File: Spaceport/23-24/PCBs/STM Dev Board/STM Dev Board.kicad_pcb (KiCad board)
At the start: 2 copper layers, 61 x 33 mm, 5 parts, among them J1 693023010811, J2 614004184726, U2 IS66WVS4M8BLL-104NLI, U3 W25X40CLSNIG

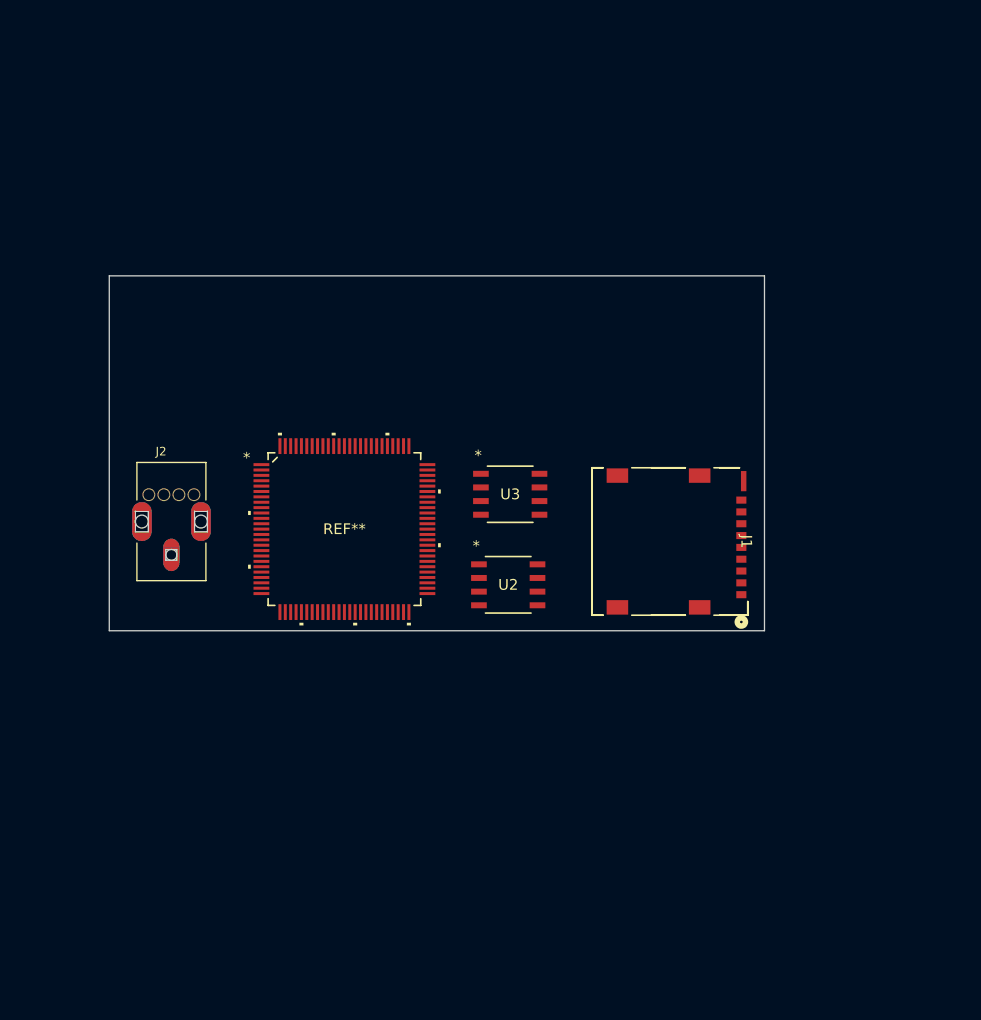
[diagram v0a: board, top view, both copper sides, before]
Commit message: commit 3
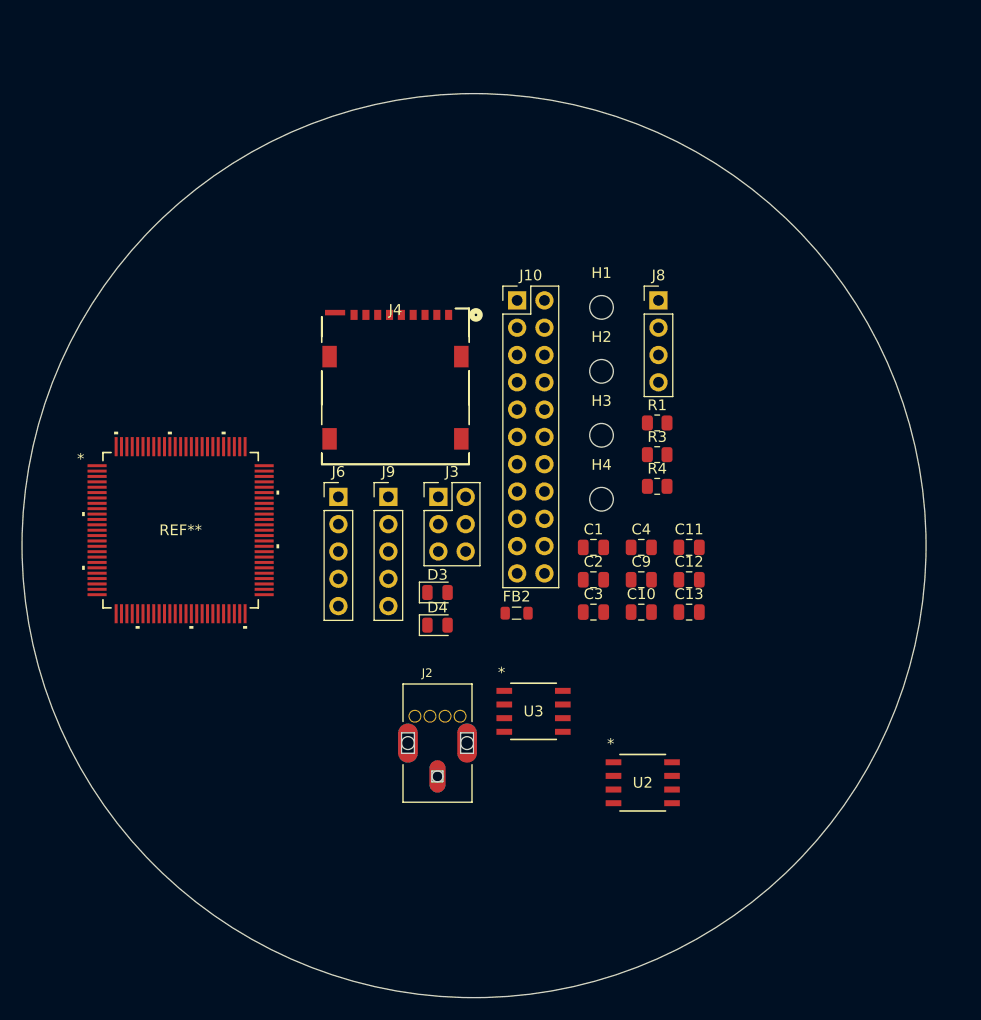
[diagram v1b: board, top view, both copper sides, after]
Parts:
- removed J1: 693023010811, 693023010811:CONN9_3010811_WRE
- removed the REF** at (137.2, 93.9)
- added C1: 100n, Capacitor_SMD:C_0805_2012Metric, F.Cu at (160.3, 95.6)
- added C10: 1u, Capacitor_SMD:C_0805_2012Metric, F.Cu at (164.8, 101.6)
- added C11: 10n, Capacitor_SMD:C_0805_2012Metric, F.Cu at (169.2, 95.6)
- added C12: 100n, Capacitor_SMD:C_0805_2012Metric, F.Cu at (169.2, 98.6)
- added C13: 1u, Capacitor_SMD:C_0805_2012Metric, F.Cu at (169.2, 101.6)
- added C2: 100n, Capacitor_SMD:C_0805_2012Metric, F.Cu at (160.3, 98.6)
- added C3: 100n, Capacitor_SMD:C_0805_2012Metric, F.Cu at (160.3, 101.6)
- added C4: 100n, Capacitor_SMD:C_0805_2012Metric, F.Cu at (164.8, 95.6)
- added C9: 1u, Capacitor_SMD:C_0805_2012Metric, F.Cu at (164.8, 98.6)
- added D3: RADIO_LED, LED_SMD:LED_0805_2012Metric, F.Cu at (145.8, 99.8)
- added D4: RADIO_LED, LED_SMD:LED_0805_2012Metric, F.Cu at (145.8, 102.8)
- added FB2: 120R, Inductor_SMD:L_0805_2012Metric, F.Cu at (153.2, 101.7)
- added H1: MountingHole, MountingHole:MountingHole_2.2mm_M2, F.Cu at (161.1, 73.2)
- added H2: MountingHole, MountingHole:MountingHole_2.2mm_M2, F.Cu at (161.1, 79.2)
- added H3: MountingHole, MountingHole:MountingHole_2.2mm_M2, F.Cu at (161.1, 85.2)
- added H4: MountingHole, MountingHole:MountingHole_2.2mm_M2, F.Cu at (161.1, 91.1)
- added J10: GPIO, Connector_PinHeader_2.54mm:PinHeader_2x11_P2.54mm_Vertical, F.Cu at (153.2, 72.6)
- added J3: SPI, Connector_PinHeader_2.54mm:PinHeader_2x03_P2.54mm_Vertical, F.Cu at (145.9, 90.9)
- added J4: 693023010811, 693023010811:CONN9_3010811_WRE, F.Cu at (146.9, 74.0)
- added J6: USART1, Connector_PinHeader_2.54mm:PinHeader_1x05_P2.54mm_Vertical, F.Cu at (136.6, 90.9)
- added J8: I2C2, Connector_PinHeader_2.54mm:PinHeader_1x04_P2.54mm_Vertical, F.Cu at (166.4, 72.6)
- added J9: USART2, Connector_PinHeader_2.54mm:PinHeader_1x05_P2.54mm_Vertical, F.Cu at (141.2, 90.9)
- added R1: 10k, Resistor_SMD:R_0805_2012Metric, F.Cu at (166.3, 84.0)
- added R3: 10k, Resistor_SMD:R_0805_2012Metric, F.Cu at (166.3, 87.0)
- added R4: 10k, Resistor_SMD:R_0805_2012Metric, F.Cu at (166.3, 89.9)
- added REF**: LQFP-100_STM, stm32h7:LQFP-100_STM-M, F.Cu at (121.9, 94.0)
- moved J2 32.2 mm to (145.8, 113.8)
- moved U2 22.3 mm to (164.9, 117.5)
- moved U3 20.3 mm to (154.8, 110.8)
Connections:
- J2 pad 1: unconnected-(J2-VBUS-Pad1) -> VBUS
- J2 pad 2: unconnected-(J2-D--Pad2) -> /USB_D-
- J2 pad 3: unconnected-(J2-D+-Pad3) -> /USB_D+
- J2 pad 4: unconnected-(J2-GND-Pad4) -> GND
- U2 pad 1: unconnected-(U2-CE#-Pad1) -> /PSram_CS
- U2 pad 2: unconnected-(U2-SO/SIO1-Pad2) -> /PSram_D0
- U2 pad 3: unconnected-(U2-SIO2-Pad3) -> /PSram_D2
- U2 pad 4: unconnected-(U2-VSS-Pad4) -> GND
- U2 pad 5: unconnected-(U2-SI/SIO0-Pad5) -> /PSram_D1
- U2 pad 6: unconnected-(U2-CLK-Pad6) -> /PSram_CLK
- U2 pad 7: unconnected-(U2-SIO3-Pad7) -> /PSram_D3
- U2 pad 8: unconnected-(U2-VDD-Pad8) -> +3.3V
- U3 pad 1: unconnected-(U3-*CS-Pad1) -> /Flash_CS
- U3 pad 2: unconnected-(U3-DO(IO1)-Pad2) -> /Flash_D0
- U3 pad 4: unconnected-(U3-GND-Pad4) -> GND
- U3 pad 5: unconnected-(U3-DI(IO0)-Pad5) -> /Flash_D1
- U3 pad 6: unconnected-(U3-CLK-Pad6) -> /Flash_CLK
- U3 pad 8: unconnected-(U3-VCC-Pad8) -> +3.3V
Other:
- board size 61 x 33 mm -> 84.1 x 84.1 mm

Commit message: main connections
all connections are made but no drc clean up has been done
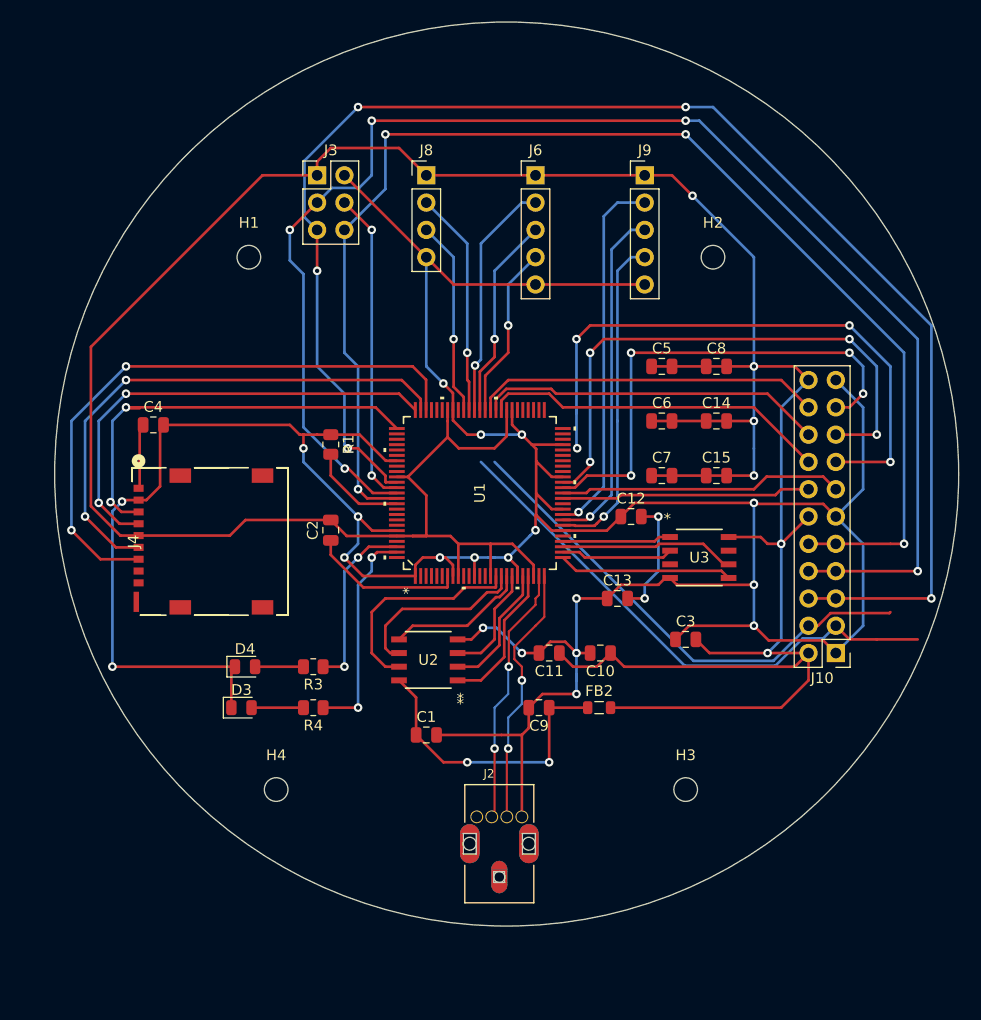
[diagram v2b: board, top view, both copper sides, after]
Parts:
- removed REF**: LQFP-100_STM, stm32h7:LQFP-100_STM-M
- added C14: 100n, Capacitor_SMD:C_0805_2012Metric, F.Cu at (171.8, 83.8)
- added C15: 100n, Capacitor_SMD:C_0805_2012Metric, F.Cu at (171.8, 88.9)
- added C5: 100n, Capacitor_SMD:C_0805_2012Metric, F.Cu at (166.7, 78.7)
- added C6: 100n, Capacitor_SMD:C_0805_2012Metric, F.Cu at (166.7, 83.8)
- added C7: 100n, Capacitor_SMD:C_0805_2012Metric, F.Cu at (166.7, 88.9)
- added C8: 100n, Capacitor_SMD:C_0805_2012Metric, F.Cu at (171.8, 78.7)
- added U1: STM32H7R3V8T6, stm32h7:LQFP-100_STM, F.Cu at (149.8, 90.5)
- D3: value RADIO_LED -> LED_USB
- D4: value RADIO_LED -> LED_SD
- moved C4 46.8 mm to (119.4, 84.2)
- moved J10 44.2 mm to (182.9, 105.4), turned to 180 degrees
- moved H4 40.6 mm to (130.8, 118.1)
- moved J9 38.3 mm to (165.1, 61.0)
- moved R4 38.0 mm to (134.3, 110.5), turned to 180 degrees
- moved R3 37.6 mm to (134.3, 106.7), turned to 180 degrees
- moved J6 35.1 mm to (154.9, 61.0)
- moved H3 33.9 mm to (168.9, 118.1)
- moved H1 33.1 mm to (128.3, 68.6)
- moved J4 33.1 mm to (118.0, 90.1), turned to 90 degrees
- moved J3 32.0 mm to (134.6, 61.0)
- moved R1 30.4 mm to (135.9, 86.0), turned to -90 degrees
- moved C2 24.9 mm to (135.9, 94.0), turned to 90 degrees
- moved J8 24.5 mm to (144.8, 61.0)
- moved C1 23.4 mm to (144.8, 113.0)
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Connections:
- J10 pad 10: /MISO -> /MOSI
- J10 pad 13: /GPIO_1 -> /GPIO_8
- J10 pad 14: /GPIO_2 -> /GPIO_4
- J10 pad 15: /GPIO_3 -> /GPIO_7
- J10 pad 16: /GPIO_4 -> /GPIO_1
- J10 pad 17: /GPIO_5 -> /GPIO_6
- J10 pad 18: /GPIO_6 -> /GPIO_2
- J10 pad 19: /GPIO_7 -> /GPIO_5
- J10 pad 20: /GPIO_8 -> /GPIO_3
- J10 pad 5: /SCLK -> /MISO
- J10 pad 6: /SCLK -> /MISO
- J10 pad 7: /MOSI -> /SCLK
- J10 pad 8: /MOSI -> /SCLK
- J10 pad 9: /MISO -> /MOSI
- J3 pad 2: /SPI_NCS -> GND
- J3 pad 4: /MOSI -> /SPI_NCS
- J3 pad 6: GND -> /MOSI
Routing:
- net +3.3V: track 0.00 -> 342.2 mm, vias 0 -> 8
- net GND: track 0.00 -> 339.0 mm, vias 0 -> 20
- net /MISO: track 0.00 -> 140.3 mm, vias 0 -> 5
- net /SCLK: track 0.00 -> 135.9 mm, vias 0 -> 5
- net /MOSI: track 0.00 -> 122.4 mm, vias 0 -> 4
- net /SCL_2: track 0.00 -> 71.5 mm, vias 0 -> 1
- net /SDA_2: track 0.00 -> 64.6 mm, vias 0 -> 1
- net /GPIO_7: track 0.00 -> 56.0 mm, vias 0 -> 4
- net /SD_Serial: track 0.00 -> 56.0 mm, vias 0 -> 2
- net /GPIO_6: track 0.00 -> 52.1 mm, vias 0 -> 4
- net /SD_CLK: track 0.00 -> 49.6 mm, vias 0 -> 2
- net /GPIO_5: track 0.00 -> 46.0 mm, vias 0 -> 4
- net /SD_Reset: track 0.00 -> 43.3 mm, vias 0 -> 2
- net /SD_Sw: track 0.00 -> 40.1 mm, vias 0 -> 2
- net /USART2_CK: track 0.00 -> 34.4 mm, vias 0 -> 1
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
